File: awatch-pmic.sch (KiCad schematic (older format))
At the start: 19 parts, among them J301 Conn_01x02, U301 MAX14690

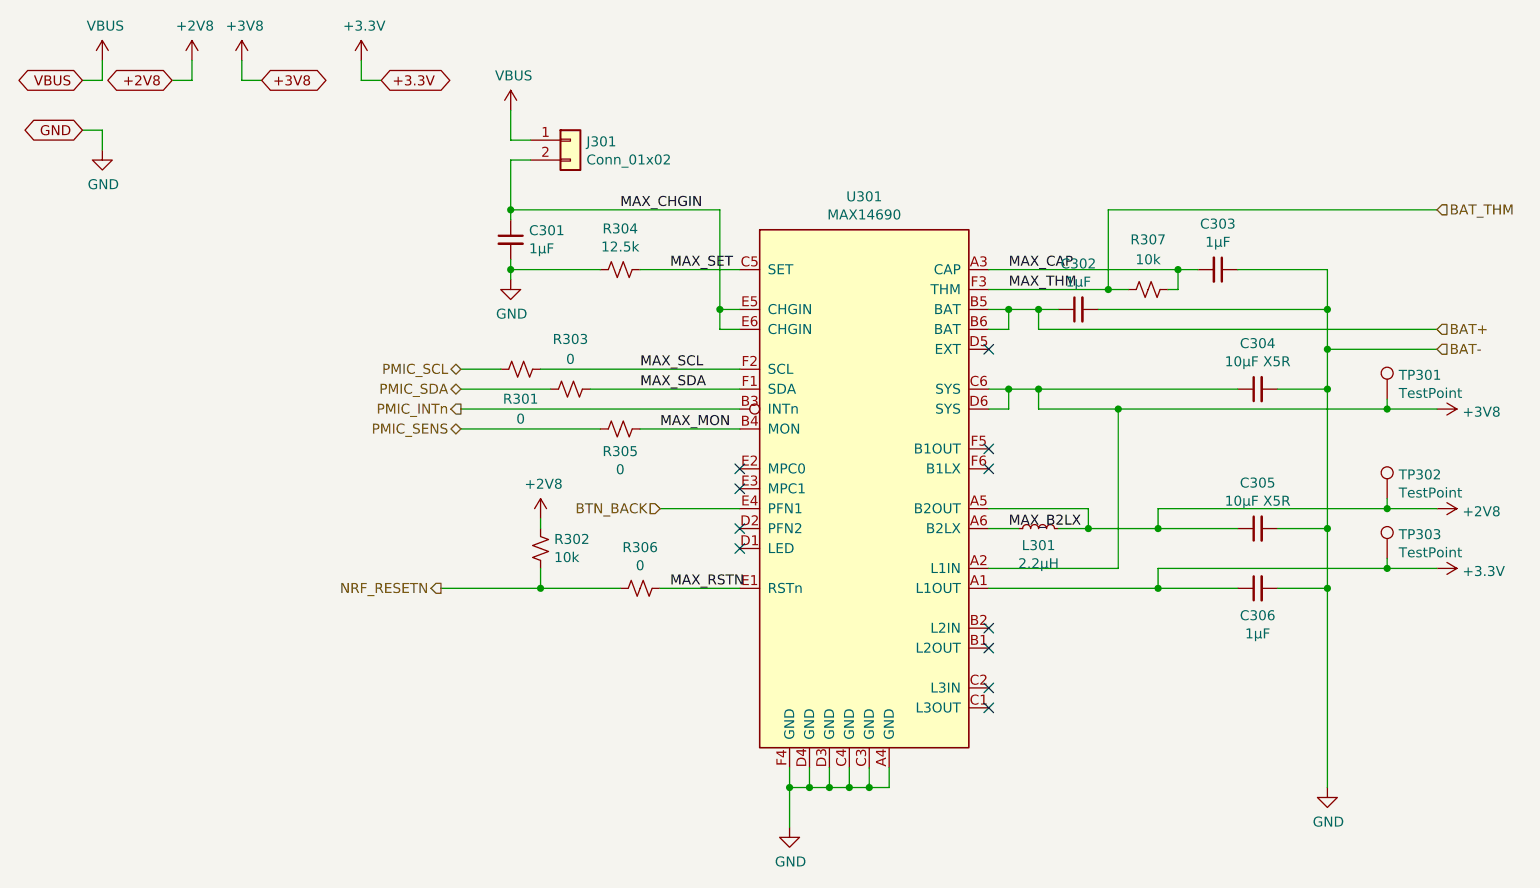
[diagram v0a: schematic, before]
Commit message: approx. final layout
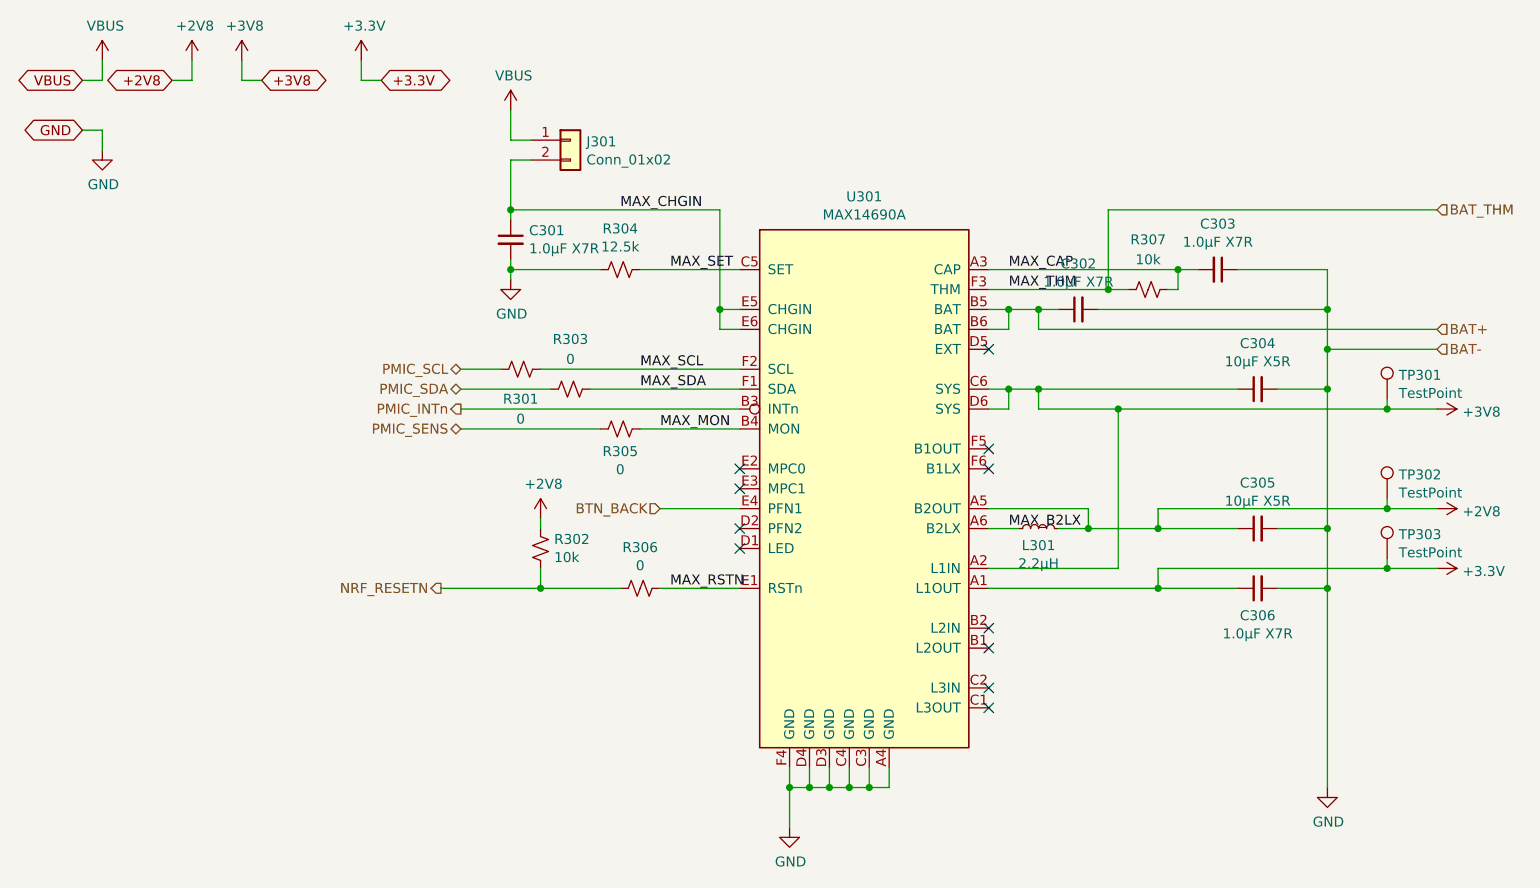
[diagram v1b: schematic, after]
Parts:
- C301, C302, C303, C306: value 1µF -> 1.0µF X7R; DigiKey PN (none) -> 1276-1946-1-ND
- C304, C305: DigiKey PN (none) -> 490-12538-1-ND
- U301: value MAX14690 -> MAX14690A; DigiKey PN (none) -> MOUSER: 700-MAX14690AEWX+
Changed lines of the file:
@@
 $Descr A4 11693 8268
 encoding utf-8
-Sheet 3 9
+Sheet 3 10
 Title "AWatch2"
 Date ""
@@
 P 3450 2050
 F 0 "C301" H 3542 2096 50  0000 L CNN
-F 1 "1µF" H 3542 2005 50  0000 L CNN
+F 1 "1.0µF X7R" H 3542 2005 50  0000 L CNN
 F 2 "Capacitor_SMD:C_0603_1608Metric" H 3450 2050 50  0001 C CNN
 F 3 "~" H 3450 2050 50  0001 C CNN
+F 4 "1276-1946-1-ND" H 0   0   50  0001 C CNN "DigiKey PN"
 	1    3450 2050
 	1    0    0    -1
@@
 P 7000 2200
 F 0 "C303" V 6771 2200 50  0000 C CNN
-F 1 "1µF" V 6862 2200 50  0000 C CNN
+F 1 "1.0µF X7R" V 6862 2200 50  0000 C CNN
 F 2 "Capacitor_SMD:C_0603_1608Metric" H 7000 2200 50  0001 C CNN
 F 3 "~" H 7000 2200 50  0001 C CNN
+F 4 "1276-1946-1-ND" H 0   0   50  0001 C CNN "DigiKey PN"
 	1    7000 2200
 	0    1    1    0
@@
 P 6300 2400
 F 0 "C302" V 6529 2400 50  0000 C CNN
-F 1 "1µF" V 6438 2400 50  0000 C CNN
+F 1 "1.0µF X7R" V 6438 2400 50  0000 C CNN
 F 2 "Capacitor_SMD:C_0603_1608Metric" H 6300 2400 50  0001 C CNN
 F 3 "~" H 6300 2400 50  0001 C CNN
+F 4 "1276-1946-1-ND" H 0   0   50  0001 C CNN "DigiKey PN"
 	1    6300 2400
 	0    -1   -1   0
@@
 F 2 "Capacitor_SMD:C_0603_1608Metric" H 7200 2800 50  0001 C CNN
 F 3 "~" H 7200 2800 50  0001 C CNN
+F 4 "490-12538-1-ND" H 0   0   50  0001 C CNN "DigiKey PN"
 	1    7200 2800
 	0    -1   -1   0
@@
 F 2 "Capacitor_SMD:C_0603_1608Metric" H 7200 3500 50  0001 C CNN
 F 3 "~" H 7200 3500 50  0001 C CNN
+F 4 "490-12538-1-ND" H 0   0   50  0001 C CNN "DigiKey PN"
 	1    7200 3500
 	0    -1   -1   0
@@
 P 4700 2000
 F 0 "U301" H 5225 2166 50  0000 C CNN
-F 1 "MAX14690" H 5225 2075 50  0000 C CNN
+F 1 "MAX14690A" H 5225 2075 50  0000 C CNN
 F 2 "awatch2-footprints:WLP-36_2.69x2.44mm_Layout6x6_P0.4mm_Ball0.22mm_Pad0.2mm_NSMD" H 4700 2000 50  0001 C CNN
 F 3 "" H 4700 2000 50  0001 C CNN
+F 4 "MOUSER: 700-MAX14690AEWX+" H 0   0   50  0001 C CNN "DigiKey PN"
 	1    4700 2000
 	1    0    0    -1
@@
 P 7200 3800
 F 0 "C306" V 7063 3800 50  0000 C CNN
-F 1 "1µF" V 6972 3800 50  0000 C CNN
+F 1 "1.0µF X7R" V 6972 3800 50  0000 C CNN
 F 2 "Capacitor_SMD:C_0603_1608Metric" H 7200 3800 50  0001 C CNN
 F 3 "~" H 7200 3800 50  0001 C CNN
+F 4 "1276-1946-1-ND" H 0   0   50  0001 C CNN "DigiKey PN"
 	1    7200 3800
 	0    -1   -1   0
